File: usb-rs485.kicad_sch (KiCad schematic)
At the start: 4 parts

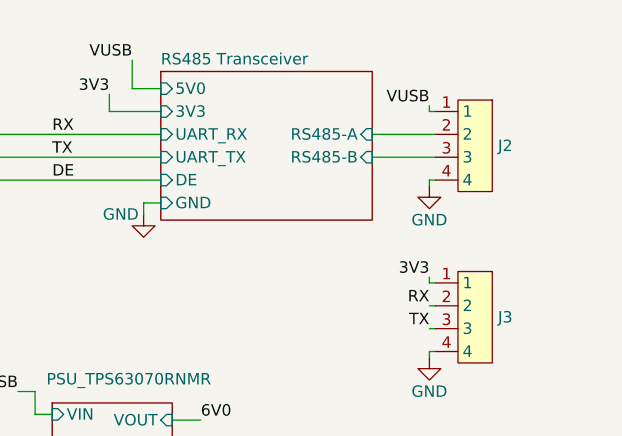
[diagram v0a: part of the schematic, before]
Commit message: moved it elsewhere but MEH
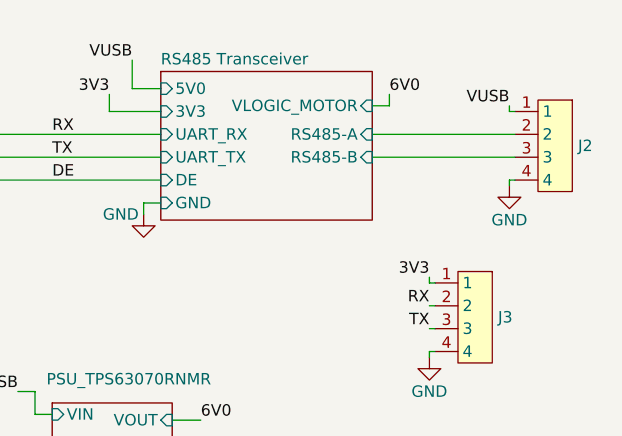
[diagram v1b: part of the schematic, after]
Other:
- sheet RS485 Transceiver ports: added VLOGIC_MOTOR; removed none
- moved on the sheet: J2
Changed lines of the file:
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@@
+    (stroke (width 0) (type default))
+  )
+  (wire (pts (xy 324.485 145.415) (xy 324.485 146.685))
     (stroke (width 0) (type default))
   )
@@
     (stroke (width 0) (type default))
   )
-  (wire (pts (xy 328.93 154.94) (xy 328.93 155.575))
+  (wire (pts (xy 337.82 154.94) (xy 337.82 155.575))
     (stroke (width 0) (type default))
   )
@@
     (stroke (width 0) (type default))
   )
-  (wire (pts (xy 322.58 149.86) (xy 329.565 149.86))
+  (wire (pts (xy 322.58 149.86) (xy 338.455 149.86))
     (stroke (width 0) (type default))
   )
@@
     (stroke (width 0) (type default))
   )
-  (wire (pts (xy 328.93 147.32) (xy 329.565 147.32))
+  (wire (pts (xy 337.82 147.32) (xy 338.455 147.32))
     (stroke (width 0) (type default))
   )
@@
     (stroke (width 0) (type default))
   )
+  (wire (pts (xy 322.58 152.4) (xy 338.455 152.4))
+    (stroke (width 0) (type default))
+  )
   (wire (pts (xy 300.355 192.405) (xy 302.26 192.405))
     (stroke (width 0) (type default))
@@
     (stroke (width 0) (type default))
   )
-  (wire (pts (xy 322.58 152.4) (xy 329.565 152.4))
-    (stroke (width 0) (type default))
-  )
   (wire (pts (xy 279.4 149.86) (xy 299.085 149.86))
     (stroke (width 0) (type default))
@@
     (stroke (width 0) (type default))
   )
-  (wire (pts (xy 328.93 146.685) (xy 328.93 147.32))
-    (stroke (width 0) (type default))
-  )
-  (wire (pts (xy 328.93 154.94) (xy 329.565 154.94))
+  (wire (pts (xy 324.485 146.685) (xy 322.58 146.685))
+    (stroke (width 0) (type default))
+  )
+  (wire (pts (xy 337.82 146.685) (xy 337.82 147.32))
+    (stroke (width 0) (type default))
+  )
+  (wire (pts (xy 337.82 154.94) (xy 338.455 154.94))
     (stroke (width 0) (type default))
   )
@@
     (effects (font (size 1.27 1.27)) (justify right bottom))
   )
+  (label "6V0" (at 324.485 145.415 0) (fields_autoplaced)
+    (effects (font (size 1.27 1.27)) (justify left bottom))
+  )
   (label "RX" (at 287.02 149.86 0) (fields_autoplaced)
     (effects (font (size 1.27 1.27)) (justify left bottom))
   )
-  (label "VUSB" (at 328.93 146.685 180) (fields_autoplaced)
+  (label "VUSB" (at 337.82 146.685 180) (fields_autoplaced)
     (effects (font (size 1.27 1.27)) (justify right bottom))
   )
@@
     )
   )
-  (symbol (lib_id "power:GND") (at 328.93 155.575 0) (unit 1)
+  (symbol (lib_id "power:GND") (at 337.82 155.575 0) (unit 1)
     (in_bom yes) (on_board yes) (dnp no)
-    (property "Reference" "#PWR011" (at 328.93 161.925 0)
-      (effects (font (size 1.27 1.27)) hide)
-    )
-    (property "Value" "GND" (at 328.93 159.385 0)
-      (effects (font (size 1.27 1.27)))
-    )
-    (property "Footprint" "" (at 328.93 155.575 0)
-      (effects (font (size 1.27 1.27)) hide)
-    )
-    (property "Datasheet" "" (at 328.93 155.575 0)
+    (property "Reference" "#PWR011" (at 337.82 161.925 0)
+      (effects (font (size 1.27 1.27)) hide)
+    )
+    (property "Value" "GND" (at 337.82 159.385 0)
+      (effects (font (size 1.27 1.27)))
+    )
+    (property "Footprint" "" (at 337.82 155.575 0)
+      (effects (font (size 1.27 1.27)) hide)
+    )
+    (property "Datasheet" "" (at 337.82 155.575 0)
       (effects (font (size 1.27 1.27)) hide)
     )
@@
     )
   )
-  (symbol (lib_id "usb-rs485:ThruHoleX4") (at 332.105 151.13 0) (mirror y) (unit 1)
+  (symbol (lib_id "usb-rs485:ThruHoleX4") (at 340.995 151.13 0) (mirror y) (unit 1)
     (in_bom no) (on_board yes) (dnp no) (fields_autoplaced)
-    (property "Reference" "J2" (at 336.55 151.13 0)
-      (effects (font (size 1.27 1.27)) (justify right))
-    )
-    (property "Value" "~" (at 330.835 149.86 0)
-      (effects (font (size 1.27 1.27)))
-    )
-    (property "Footprint" "usb-rs485:ThruHoleBreadboardX4" (at 330.835 149.86 0)
-      (effects (font (size 1.27 1.27)) hide)
-    )
-    (property "Datasheet" "" (at 330.835 149.86 0)
+    (property "Reference" "J2" (at 345.44 151.13 0)
+      (effects (font (size 1.27 1.27)) (justify right))
+    )
+    (property "Value" "~" (at 339.725 149.86 0)
+      (effects (font (size 1.27 1.27)))
+    )
+    (property "Footprint" "usb-rs485:ThruHoleBreadboardX4" (at 339.725 149.86 0)
+      (effects (font (size 1.27 1.27)) hide)
+    )
+    (property "Datasheet" "" (at 339.725 149.86 0)
       (effects (font (size 1.27 1.27)) hide)
     )
@@
       (effects (font (size 1.27 1.27)) (justify right))
     )
+    (pin "VLOGIC_MOTOR" input (at 322.58 146.685 0)
+      (effects (font (size 1.27 1.27)) (justify right))
+    )
